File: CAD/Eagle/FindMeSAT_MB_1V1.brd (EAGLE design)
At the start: 99 x 49.2 mm, 135 parts, among them Q101 ABS07-32.768KHZ, Q651 ABM3B-16MHZ-10-R50-1-U, U1001 CFPT-141-20MHZ, U101 ATXMEGA256A3BU-AU, U1011 OPA354, U1021 OPA354, U1111 LM2831YMF, U1121 LM4120IM5-3.0, U201 SIM808, U301 MPU-9250, U401 MS5607-02BA03, U501 SHT31-DIS, U601 AX5243, X111 AVR-JTAG-10, X121 MOLEX_90130_2X03, X131 HEADER-2X3, X181 HEADER-2X3, X291 MCX-J-P-X-RA-SM1, X685 SMA_CON, X701 MOLEX_105017-0001, X801 MICROSIM-8P_SDCARD-8P_MOLEX-1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, X901 JST_S3B-XH-A

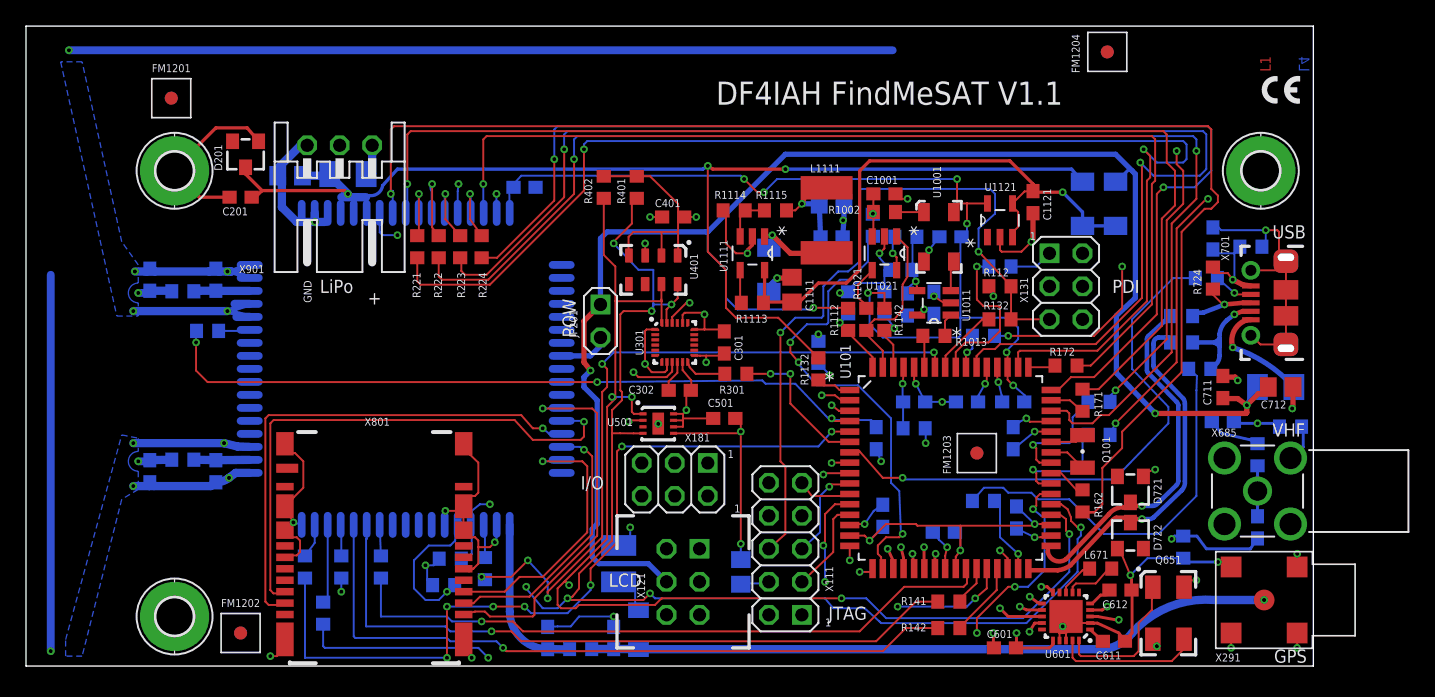
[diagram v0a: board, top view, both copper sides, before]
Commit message: CAD/Docs - V1.1 reworked to conform to PCB house Smart-Prototyping
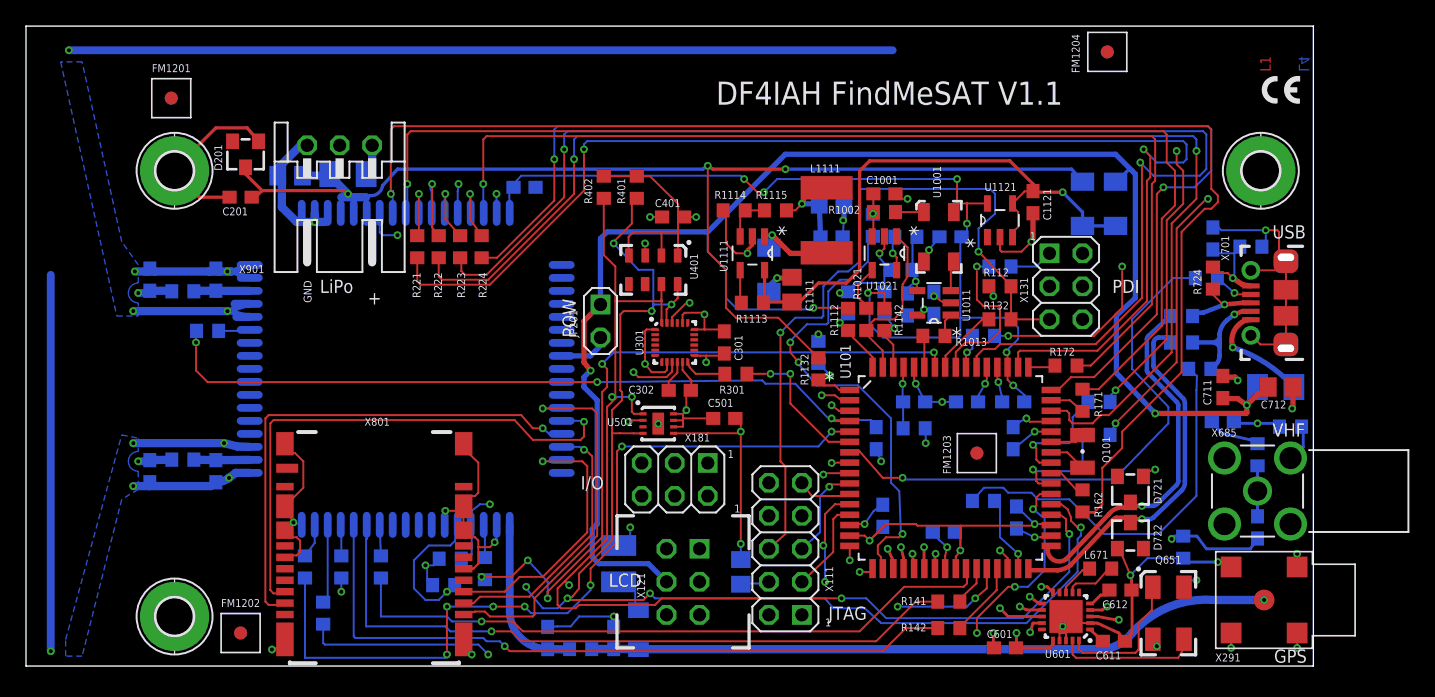
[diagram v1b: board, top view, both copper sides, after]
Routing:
- net GND: track 234.3 -> 232.4 mm
- net CLK16P: track 11.2 -> 10.7 mm
